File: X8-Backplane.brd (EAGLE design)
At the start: 122.1 x 122.1 mm, 17 parts

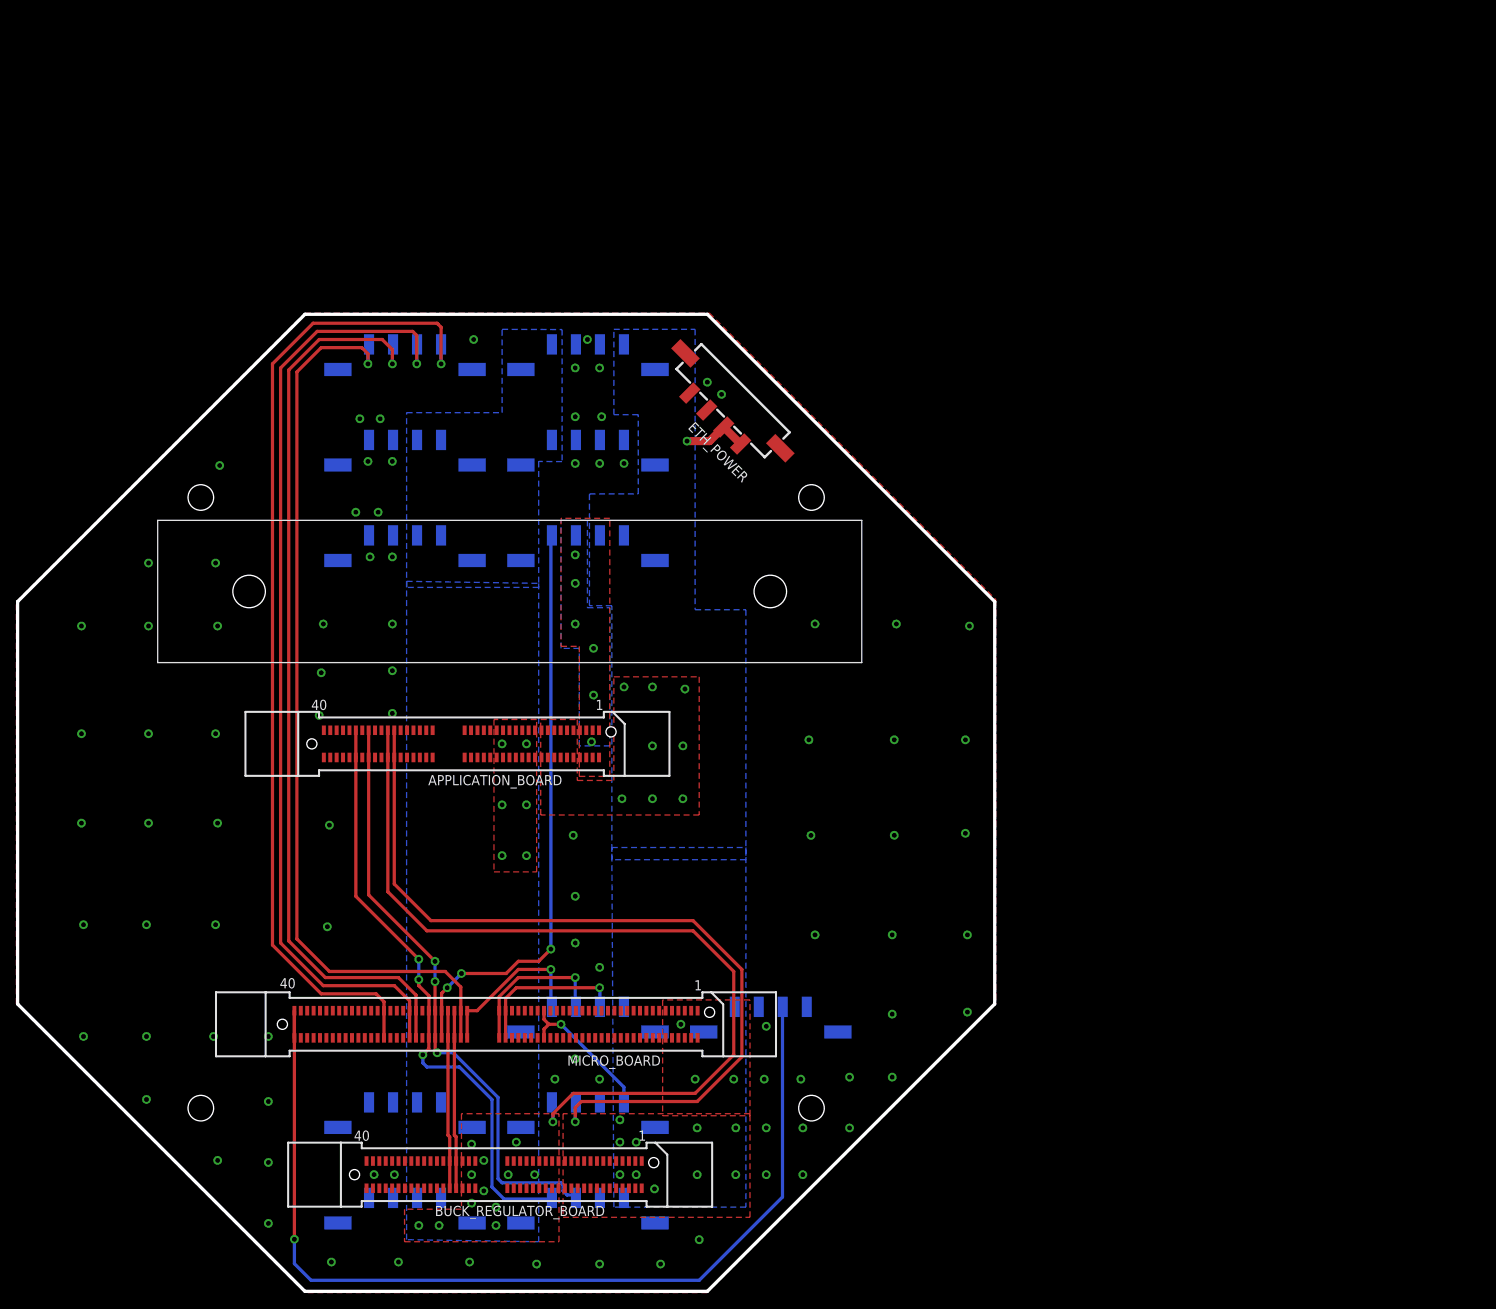
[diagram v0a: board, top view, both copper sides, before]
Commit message: Moved the board into a valid location
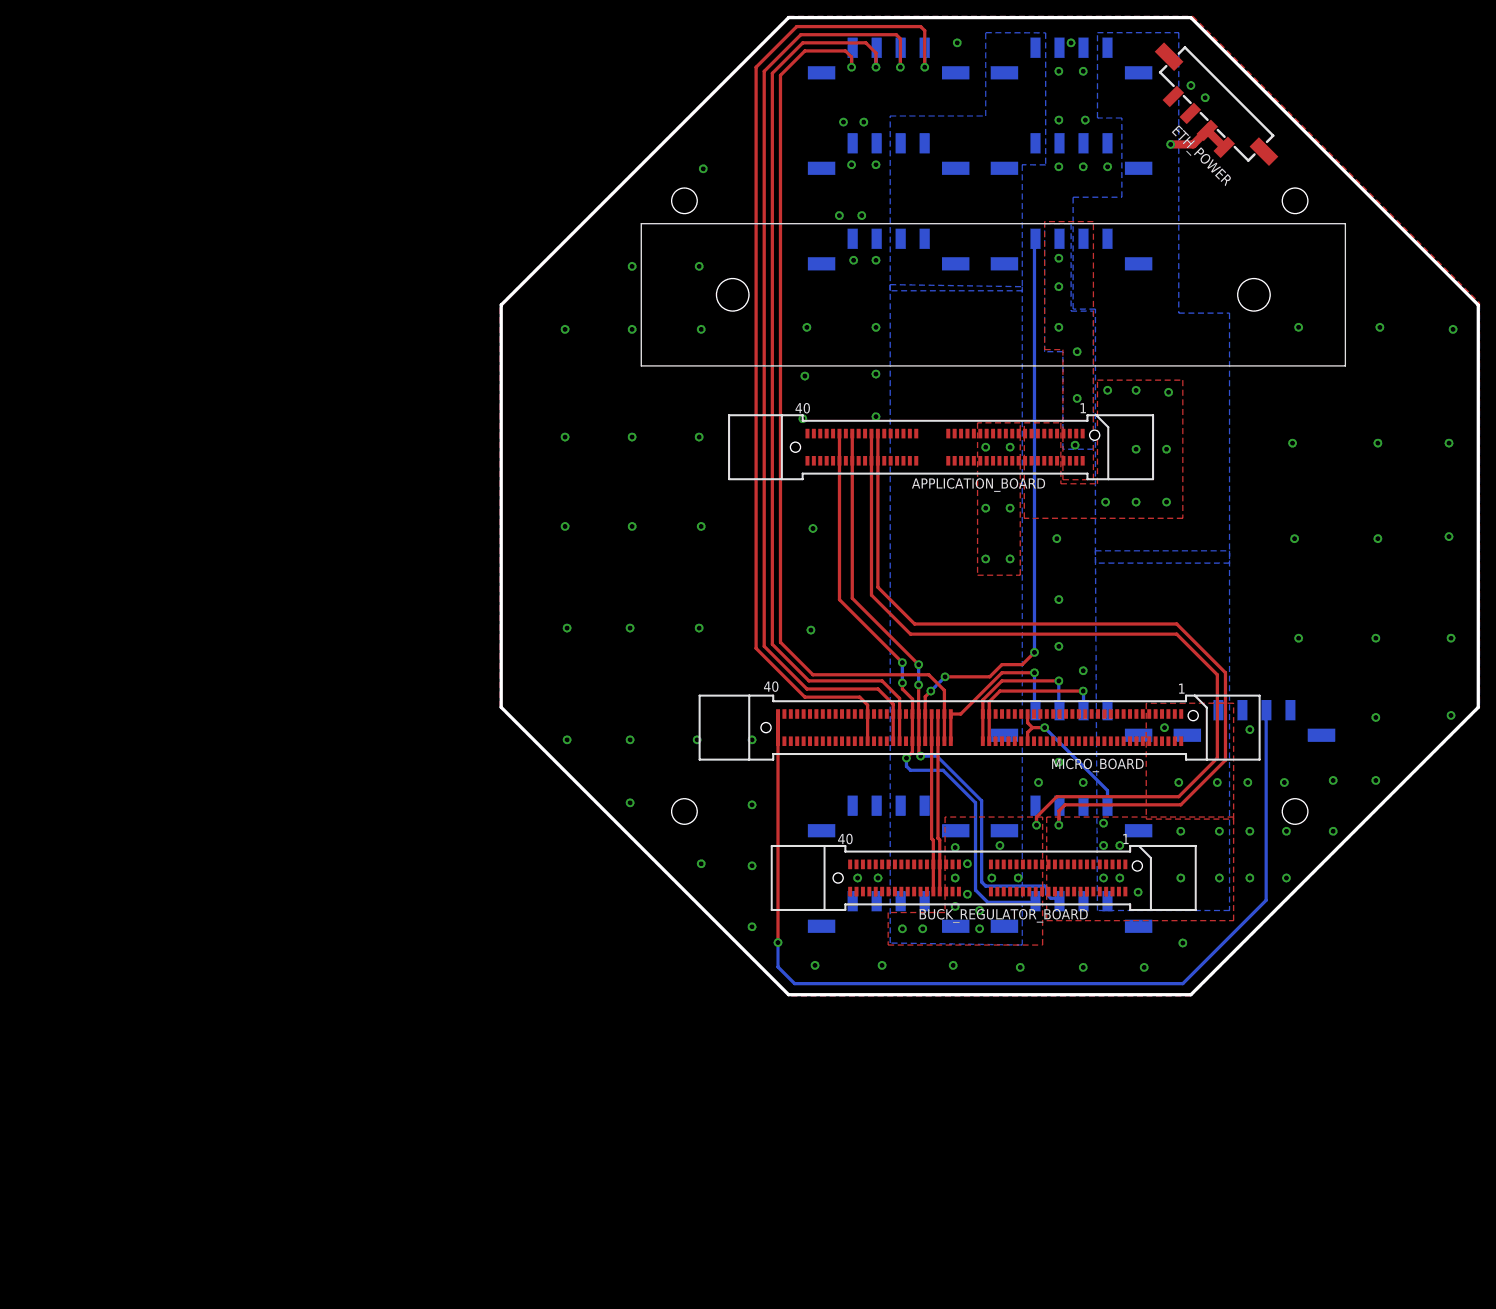
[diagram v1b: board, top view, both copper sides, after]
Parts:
- moved APPLICATION_BOARD 70.9 mm to (54.9, 44.5)
- moved BRICKS_COM 70.9 mm to (80.8, -16.3)
- moved BUCK_REGULATOR_BOARD 70.9 mm to (60.2, -9.40)
- moved ETH_POWER 70.9 mm to (96.5, 80.8)
- moved EXTRA_SERVO 70.9 mm to (103.6, 7.62)
- moved MAIN_CAM_DATA 70.9 mm to (80.8, 66.5)
- moved MAIN_CAM_POW 70.9 mm to (80.8, 78.5)
- moved MICRO_BOARD 70.9 mm to (59.2, 9.40)
- moved NAV_COM 70.9 mm to (57.9, 90.4)
- moved NAV_POWER 70.9 mm to (80.8, 90.4)
- moved POWER_INPUT 70.9 mm to (57.9, -16.3)
- moved SEC_CAM_1 70.9 mm to (57.9, 78.5)
- moved SEC_CAM_2 70.9 mm to (57.9, 66.5)
- moved SOLENOID_DATA 70.9 mm to (80.8, 7.62)
- moved SOLENOID_POWER 70.9 mm to (57.9, -4.32)
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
